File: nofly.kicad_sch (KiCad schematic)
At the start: 8 parts, among them J1 USB_C_Receptacle_USB2.0_16P, J2 Conn_01x04, U1 USBLC6-2P6

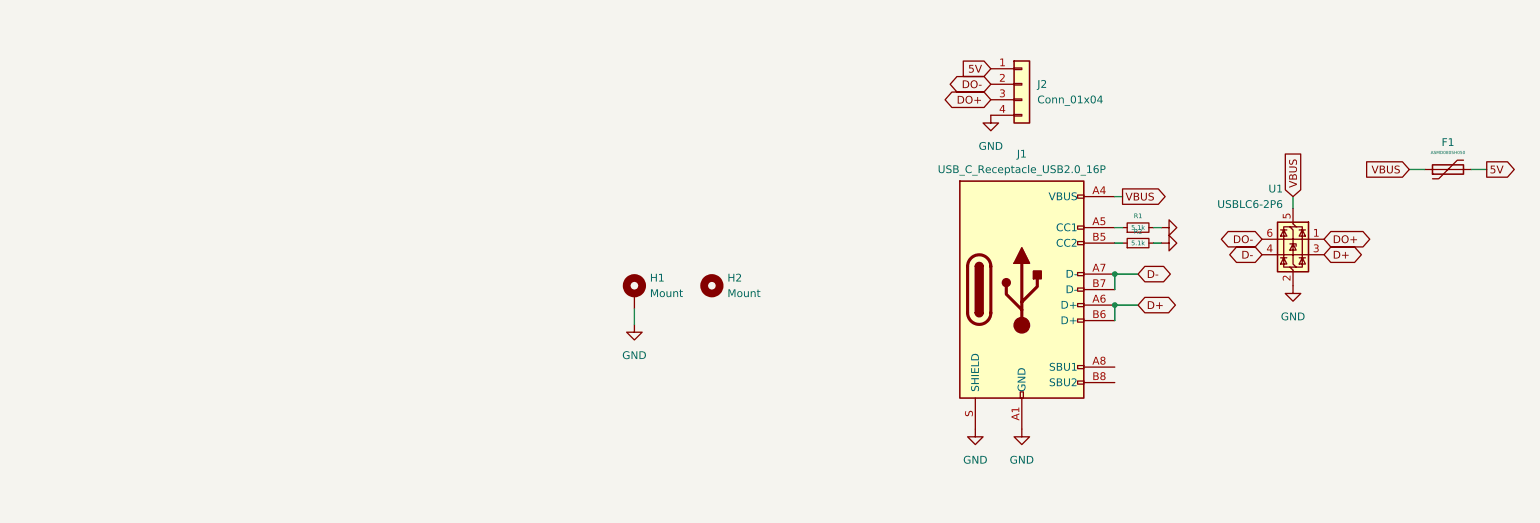
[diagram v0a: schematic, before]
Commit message: Organize schematic
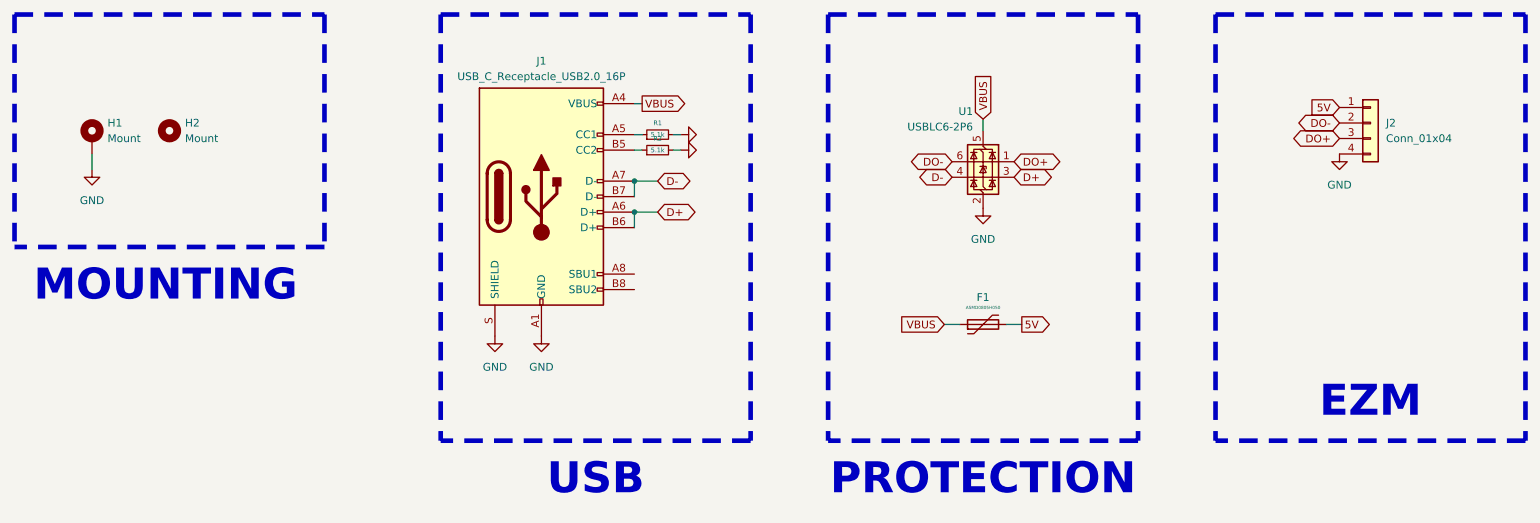
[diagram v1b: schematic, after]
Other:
- note added: "EZM"
- note added: "MOUNTING"
- note added: "PROTECTION"
- note added: "USB"
- moved on the sheet: F1, H1, H2, J1, J2, R1, R2, U1
